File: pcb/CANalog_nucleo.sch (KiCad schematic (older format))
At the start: 74 parts, among them J1 USB_B_Micro, J2 PWR, J3 ESP_PROG, J5 AOUT, J6 DSUB9_Male, Q1 DMP3099L-7, Q2 MMBT2222A, SW1 SW_Push, SW2 SW_Push, U1 NUCLEO64-F302R8, U2 BL9342, U3 MCP6002-xSN, U4 SN65HVD230, U5 ESP-12E, U6 OPA330xxDBV, U7 74AHC1G66

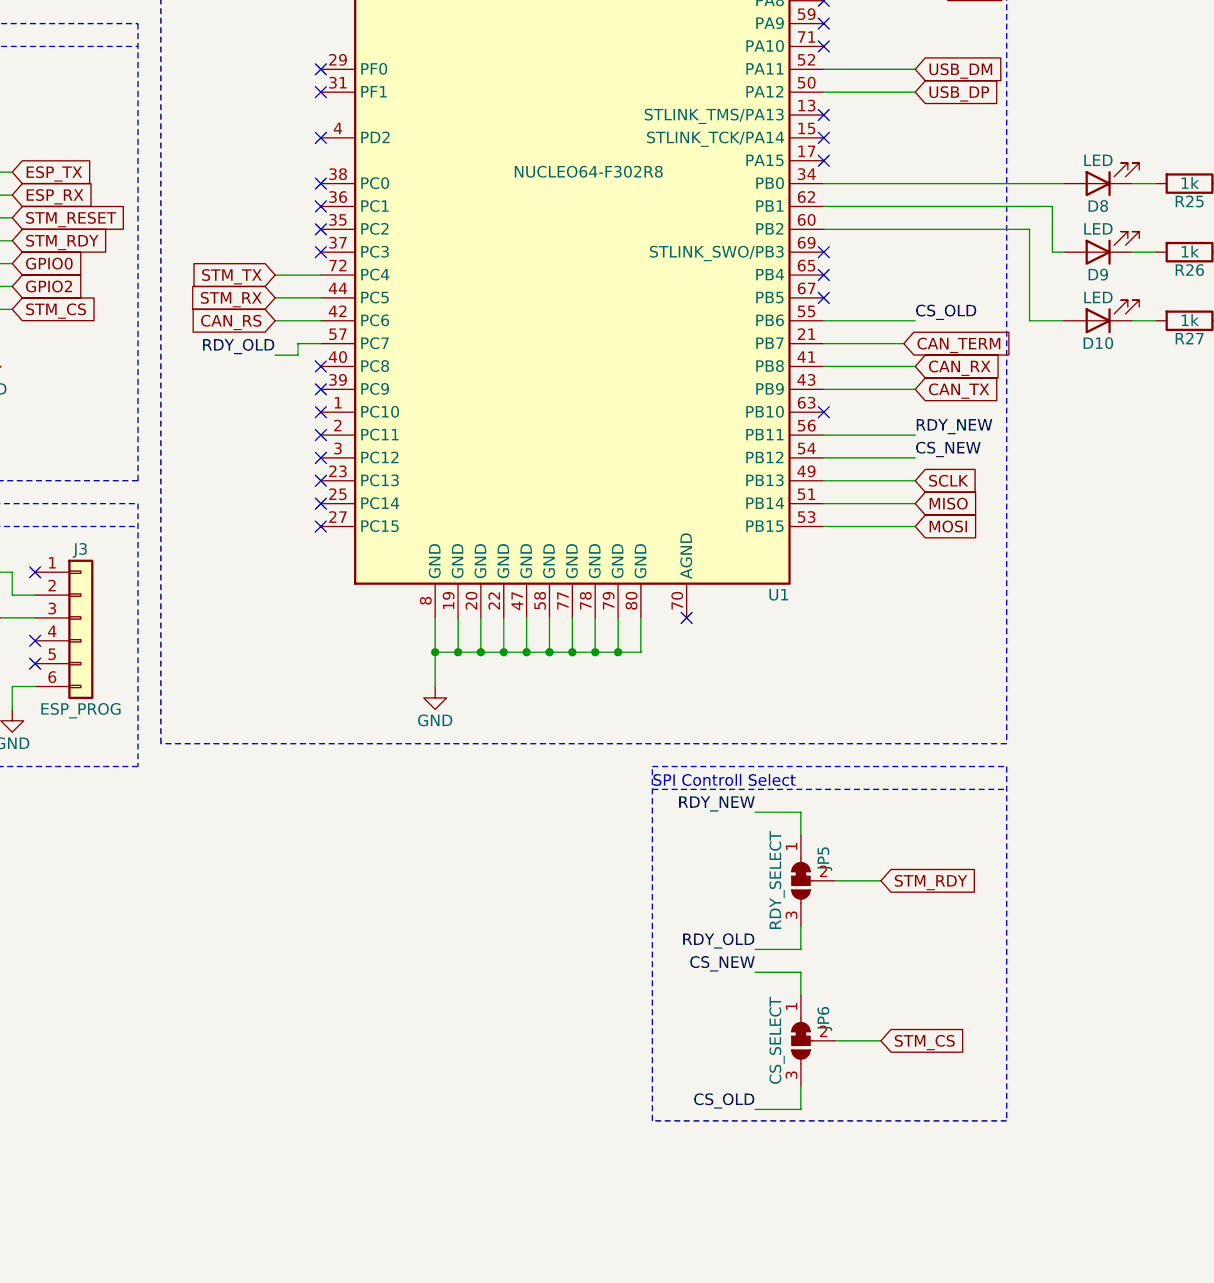
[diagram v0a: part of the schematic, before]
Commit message: start new pcb layout
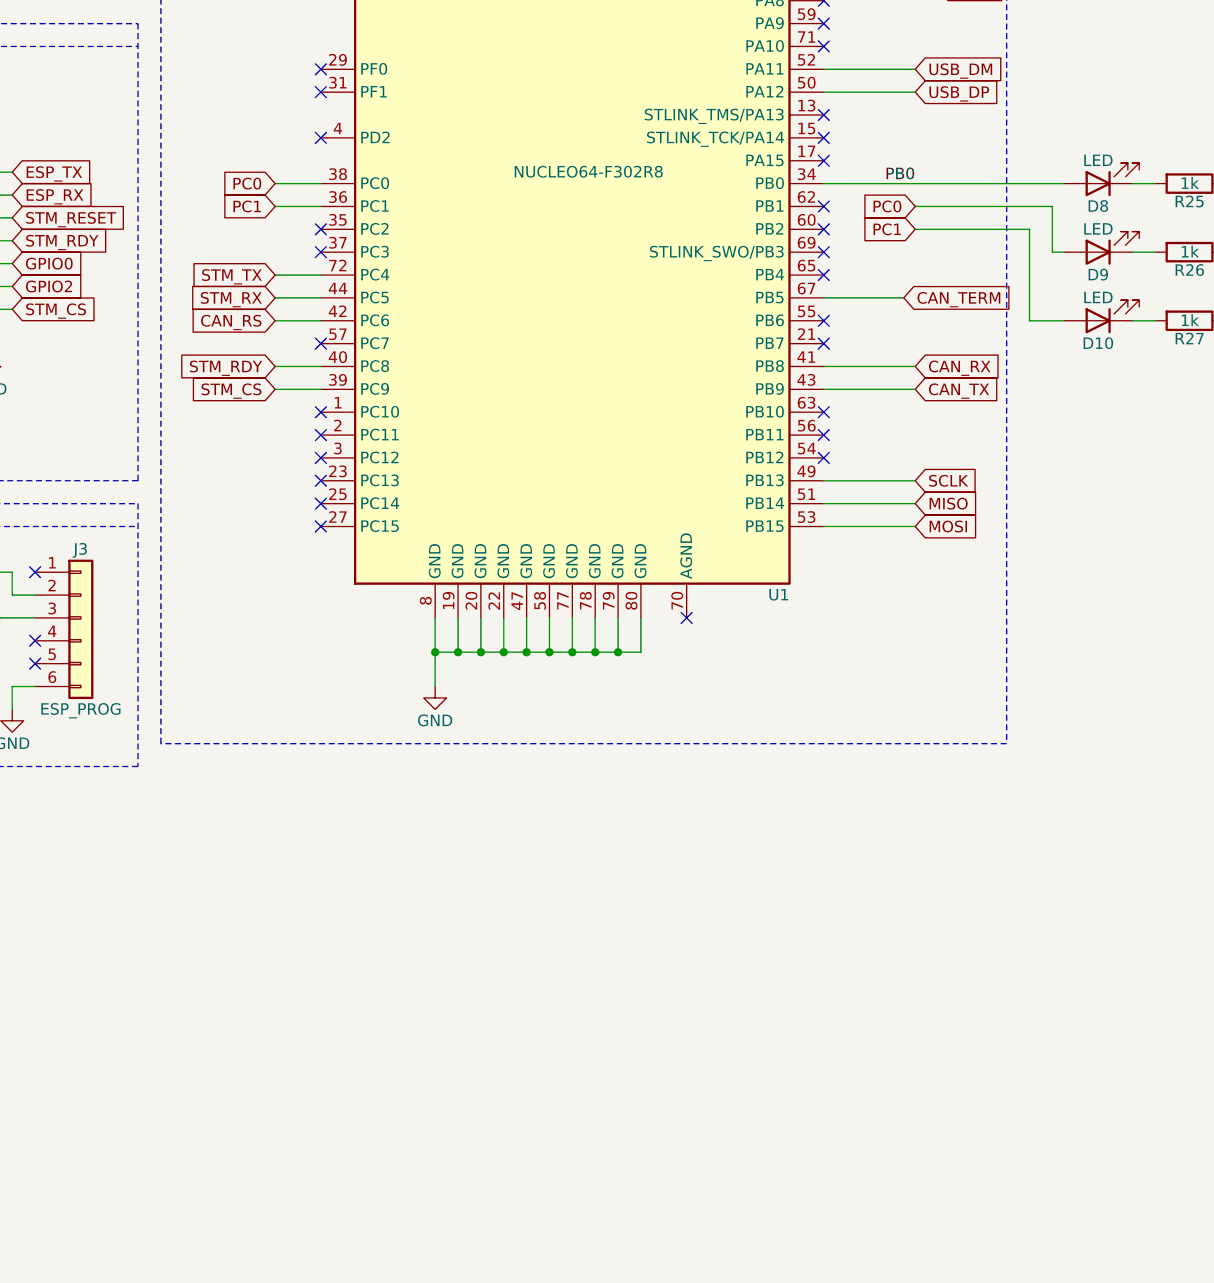
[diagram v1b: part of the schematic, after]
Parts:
- removed JP5: RDY_SELECT, Jumper:SolderJumper-3_P1.3mm_Bridged12_RoundedPad1.0x1.5mm, symbol Jumper:SolderJumper_3_Bridged12
- removed JP6: CS_SELECT, Jumper:SolderJumper-3_P1.3mm_Bridged12_RoundedPad1.0x1.5mm, symbol Jumper:SolderJumper_3_Bridged12
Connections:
- net CAN_TERM: now also U1.67 (PB5); no longer U1.21 (PB7)
- net STM_CS: now also U1.39 (PC9)
- net STM_RDY: now also U1.40 (PC8)
- net PB0: now reaches D8.2 (A), U1.34 (PB0)
- net PC1: now reaches U1.36 (PC1)
- net PC1: now also D10.2 (A)
- net PC0: now reaches U1.38 (PC0)
- net PC0: now also D9.2 (A)
- net at U1.60 (PB2): no longer D10.2 (A)
- net at U1.62 (PB1): no longer D9.2 (A)
- net CS_NEW: no longer names the net of U1.54 (PB12)
- net CS_OLD: no longer names the net of U1.55 (PB6)
- net RDY_NEW: no longer names the net of U1.56 (PB11)
- net RDY_OLD: no longer names the net of U1.57 (PC7)
- no-connect marks 57 -> 59
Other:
- note removed: "SPI Controll Select"
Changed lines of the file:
@@
 NoConn ~ 9000 5350
 NoConn ~ 9000 5450
-NoConn ~ 9000 5550
 NoConn ~ 9000 6050
 NoConn ~ 8400 6950
@@
 NoConn ~ 6800 6150
 NoConn ~ 6800 6050
-NoConn ~ 6800 5950
-NoConn ~ 6800 5850
 NoConn ~ 6800 5350
 NoConn ~ 6800 4850
@@
 Wire Wire Line
 	6600 3550 6700 3550
-Wire Wire Line
-	9000 5650 9400 5650
-Wire Wire Line
-	9000 6250 9400 6250
-Text Label 9400 6250 0    50   ~ 0
-CS_NEW
-Text Label 9400 5650 0    50   ~ 0
-CS_OLD
-Text Label 6600 5800 2    50   ~ 0
-RDY_OLD
-Text Label 9400 6150 0    50   ~ 0
-RDY_NEW
-Wire Wire Line
-	9000 6150 9400 6150
-Wire Wire Line
-	6800 5750 6700 5750
-Wire Wire Line
-	6700 5750 6700 5800
-Wire Wire Line
-	6700 5800 6600 5800
 $Comp
 L Device:Jumper_NO_Small JP4
@@
 Wire Wire Line
 	16150 3150 16150 3050
-Text GLabel 9350 5750 2    50   Input ~ 0
+Text GLabel 9350 5550 2    50   Input ~ 0
 CAN_TERM
-Wire Wire Line
-	9350 5750 9000 5750
 Text GLabel 14300 2950 0    50   Input ~ 0
 CAN_TERM
@@
 Wire Wire Line
 	5800 1100 5800 950
-Text GLabel 9250 8800 2    50   Input ~ 0
+Text GLabel 6600 5950 0    50   Input ~ 0
 STM_CS
-Text GLabel 9250 8100 2    50   Input ~ 0
-STM_RDY
-$Comp
-L Jumper:SolderJumper_3_Bridged12 JP5
-U 1 1 6087F94F
-P 8900 8100
-F 0 "JP5" H 8800 8000 50  0000 C CNN
-F 1 "RDY_SELECT" H 8900 8210 50  0000 C CNN
-F 2 "Jumper:SolderJumper-3_P1.3mm_Bridged12_RoundedPad1.0x1.5mm" H 8900 8100 50  0001 C CNN
-F 3 "~" H 8900 8100 50  0001 C CNN
-	1    8900 8100
-	0    -1   1    0
-$EndComp
-$Comp
-L Jumper:SolderJumper_3_Bridged12 JP6
-U 1 1 60881304
-P 8900 8800
-F 0 "JP6" H 8800 8700 50  0000 C CNN
-F 1 "CS_SELECT" H 8900 8910 50  0000 C CNN
-F 2 "Jumper:SolderJumper-3_P1.3mm_Bridged12_RoundedPad1.0x1.5mm" H 8900 8800 50  0001 C CNN
-F 3 "~" H 8900 8800 50  0001 C CNN
-	1    8900 8800
-	0    -1   1    0
-$EndComp
-Wire Wire Line
-	9250 8800 9050 8800
-Wire Wire Line
-	9250 8100 9050 8100
-Text Label 8700 7800 2    50   ~ 0
-RDY_NEW
-Wire Wire Line
-	8700 7800 8900 7800
-Wire Wire Line
-	8900 7800 8900 7900
-Text Label 8700 8400 2    50   ~ 0
-RDY_OLD
-Wire Wire Line
-	8700 8400 8900 8400
-Wire Wire Line
-	8900 8400 8900 8300
-Text Label 8700 9100 2    50   ~ 0
-CS_OLD
-Wire Wire Line
-	8700 9100 8900 9100
-Wire Wire Line
-	8900 9100 8900 9000
-Text Label 8700 8500 2    50   ~ 0
-CS_NEW
-Wire Wire Line
-	8700 8500 8900 8500
-Wire Wire Line
-	8900 8500 8900 8600
-Text Notes 8250 7700 0    50   ~ 0
-SPI Controll Select
-Wire Notes Line
-	8250 7700 9800 7700
-Wire Notes Line
-	9800 9150 8250 9150
-Wire Notes Line
-	8250 9150 8250 7600
-Wire Notes Line
-	8250 7600 9800 7600
-Wire Notes Line
-	9800 7600 9800 9150
 NoConn ~ 9000 4950
-NoConn ~ 6800 5050
-NoConn ~ 6800 5150
 NoConn ~ 6800 5250
 NoConn ~ 9000 3450
@@
 $EndComp
 $Comp
+L Device:R R25
+U 1 1 635EBB6A
+P 10600 5050
+F 0 "R25" V 10680 5050 50  0000 C CNN
+F 1 "1k" V 10600 5050 50  0000 C CNN
+F 2 "Resistor_SMD:R_0805_2012Metric" V 10530 5050 50  0001 C CNN
+F 3 "~" H 10600 5050 50  0001 C CNN
+	1    10600 5050
+	0    1    1    0
+$EndComp
+$Comp
+L Device:LED D8
+U 1 1 635F6452
+P 10200 5050
+F 0 "D8" H 10200 5150 50  0000 C CNN
+F 1 "LED" H 10200 4950 50  0000 C CNN
+F 2 "LED_SMD:LED_0603_1608Metric" H 10200 5050 50  0001 C CNN
+F 3 "~" H 10200 5050 50  0001 C CNN
+	1    10200 5050
+	-1   0    0    1
+$EndComp
+$Comp
+L Device:LED D10
+U 1 1 635F6B4D
+P 10200 5650
+F 0 "D10" H 10200 5750 50  0000 C CNN
+F 1 "LED" H 10200 5550 50  0000 C CNN
+F 2 "LED_SMD:LED_0603_1608Metric" H 10200 5650 50  0001 C CNN
+F 3 "~" H 10200 5650 50  0001 C CNN
+	1    10200 5650
+	-1   0    0    1
+$EndComp
+$Comp
+L Device:R R27
+U 1 1 63627AF7
+P 10600 5650
+F 0 "R27" V 10680 5650 50  0000 C CNN
+F 1 "1k" V 10600 5650 50  0000 C CNN
+F 2 "Resistor_SMD:R_0805_2012Metric" V 10530 5650 50  0001 C CNN
+F 3 "~" H 10600 5650 50  0001 C CNN
+	1    10600 5650
+	0    1    1    0
+$EndComp
+$Comp
+L power:GND #PWR050
+U 1 1 63628CEC
+P 10950 5850
+F 0 "#PWR050" H 10950 5600 50  0001 C CNN
+F 1 "GND" H 10950 5700 50  0000 C CNN
+F 2 "" H 10950 5850 50  0001 C CNN
+F 3 "" H 10950 5850 50  0001 C CNN
+	1    10950 5850
+	1    0    0    -1
+$EndComp
+Wire Wire Line
+	10750 5050 10950 5050
+Wire Wire Line
+	10750 5650 10950 5650
+Wire Wire Line
+	10950 5650 10950 5850
+Wire Wire Line
+	10450 5050 10350 5050
+Wire Wire Line
+	10450 5650 10350 5650
+Wire Wire Line
+	10050 5050 9000 5050
+$Comp
+L Device:R R28
+U 1 1 63887C0E
+P 2650 3700
+F 0 "R28" V 2730 3700 50  0000 C CNN
+F 1 "20k" V 2650 3700 50  0000 C CNN
+F 2 "Resistor_SMD:R_0805_2012Metric" V 2580 3700 50  0001 C CNN
+F 3 "~" H 2650 3700 50  0001 C CNN
+	1    2650 3700
+	1    0    0    -1
+$EndComp
+Wire Wire Line
+	2650 3550 2650 3500
+Text GLabel 6600 5850 0    50   Input ~ 0
+STM_RDY
+Wire Wire Line
+	6600 5850 6800 5850
+NoConn ~ 6800 5750
+Wire Wire Line
+	6600 5950 6800 5950
+NoConn ~ 9000 5650
+NoConn ~ 9000 6150
+NoConn ~ 9000 6250
+Wire Wire Line
+	9000 5550 9350 5550
+NoConn ~ 9000 5750
+Wire Wire Line
+	10450 5350 10350 5350
+Wire Wire Line
+	10750 5350 10950 5350
+$Comp
+L Device:R R26
+U 1 1 636274C8
+P 10600 5350
+F 0 "R26" V 10680 5350 50  0000 C CNN
+F 1 "1k" V 10600 5350 50  0000 C CNN
+F 2 "Resistor_SMD:R_0805_2012Metric" V 10530 5350 50  0001 C CNN
+F 3 "~" H 10600 5350 50  0001 C CNN
+	1    10600 5350
+	0    1    1    0
+$EndComp
+$Comp
 L Device:LED D9
 U 1 1 635E736D
@@
 	-1   0    0    1
 $EndComp
-$Comp
-L Device:R R25
-U 1 1 635EBB6A
-P 10600 5050
-F 0 "R25" V 10680 5050 50  0000 C CNN
-F 1 "1k" V 10600 5050 50  0000 C CNN
-F 2 "Resistor_SMD:R_0805_2012Metric" V 10530 5050 50  0001 C CNN
-F 3 "~" H 10600 5050 50  0001 C CNN
-	1    10600 5050
-	0    1    1    0
-$EndComp
-$Comp
-L Device:LED D8
-U 1 1 635F6452
-P 10200 5050
-F 0 "D8" H 10200 5150 50  0000 C CNN
-F 1 "LED" H 10200 4950 50  0000 C CNN
-F 2 "LED_SMD:LED_0603_1608Metric" H 10200 5050 50  0001 C CNN
-F 3 "~" H 10200 5050 50  0001 C CNN
-	1    10200 5050
-	-1   0    0    1
-$EndComp
-$Comp
-L Device:LED D10
-U 1 1 635F6B4D
-P 10200 5650
-F 0 "D10" H 10200 5750 50  0000 C CNN
-F 1 "LED" H 10200 5550 50  0000 C CNN
-F 2 "LED_SMD:LED_0603_1608Metric" H 10200 5650 50  0001 C CNN
-F 3 "~" H 10200 5650 50  0001 C CNN
-	1    10200 5650
-	-1   0    0    1
-$EndComp
-$Comp
-L Device:R R26
-U 1 1 636274C8
-P 10600 5350
-F 0 "R26" V 10680 5350 50  0000 C CNN
-F 1 "1k" V 10600 5350 50  0000 C CNN
-F 2 "Resistor_SMD:R_0805_2012Metric" V 10530 5350 50  0001 C CNN
-F 3 "~" H 10600 5350 50  0001 C CNN
-	1    10600 5350
-	0    1    1    0
-$EndComp
-$Comp
-L Device:R R27
-U 1 1 63627AF7
-P 10600 5650
-F 0 "R27" V 10680 5650 50  0000 C CNN
-F 1 "1k" V 10600 5650 50  0000 C CNN
-F 2 "Resistor_SMD:R_0805_2012Metric" V 10530 5650 50  0001 C CNN
-F 3 "~" H 10600 5650 50  0001 C CNN
-	1    10600 5650
-	0    1    1    0
-$EndComp
-$Comp
-L power:GND #PWR050
-U 1 1 63628CEC
-P 10950 5850
-F 0 "#PWR050" H 10950 5600 50  0001 C CNN
-F 1 "GND" H 10950 5700 50  0000 C CNN
-F 2 "" H 10950 5850 50  0001 C CNN
-F 3 "" H 10950 5850 50  0001 C CNN
-	1    10950 5850
-	1    0    0    -1
-$EndComp
-Wire Wire Line
-	10750 5050 10950 5050
 Wire Wire Line
 	10950 5050 10950 5350
-Wire Wire Line
-	10750 5650 10950 5650
 Connection ~ 10950 5650
-Wire Wire Line
-	10950 5650 10950 5850
-Wire Wire Line
-	10750 5350 10950 5350
 Connection ~ 10950 5350
 Wire Wire Line
 	10950 5350 10950 5650
-Wire Wire Line
-	10450 5050 10350 5050
-Wire Wire Line
-	10450 5350 10350 5350
-Wire Wire Line
-	10450 5650 10350 5650
-Wire Wire Line
-	10050 5050 9000 5050
-Wire Wire Line
-	9000 5150 10000 5150
+Text Label 9400 5050 2    50   ~ 0
+PB0
+Text GLabel 6600 5050 0    50   Input ~ 0
+PC0
+Text GLabel 6600 5150 0    50   Input ~ 0
+PC1
+Wire Wire Line
+	6600 5050 6800 5050
+Wire Wire Line
+	6600 5150 6800 5150
+Text GLabel 9400 5150 0    50   Input ~ 0
+PC0
+Text GLabel 9400 5250 0    50   Input ~ 0
+PC1
+Wire Wire Line
+	9400 5150 10000 5150
 Wire Wire Line
 	10000 5150 10000 5350
@@
 	9900 5650 9900 5250
 Wire Wire Line
-	9900 5250 9000 5250
-$Comp
-L Device:R R28
-U 1 1 63887C0E
-P 2650 3700
-F 0 "R28" V 2730 3700 50  0000 C CNN
-F 1 "20k" V 2650 3700 50  0000 C CNN
-F 2 "Resistor_SMD:R_0805_2012Metric" V 2580 3700 50  0001 C CNN
-F 3 "~" H 2650 3700 50  0001 C CNN
-	1    2650 3700
-	1    0    0    -1
-$EndComp
-Wire Wire Line
-	2650 3550 2650 3500
+	9900 5250 9400 5250
+NoConn ~ 9000 5150
+NoConn ~ 9000 5250
 $EndSCHEMATC
